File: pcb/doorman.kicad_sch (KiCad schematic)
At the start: 58 parts, among them J1 USB-C Connector, J2 Screw Terminals, J3 3V3 Test Pad, J4 Extension Board Connector, J5 Siedle BUS RX Test Pad, J6 BUS Test Pad, J7 BUS RX Test Pad, J8 TX Test Pad, J9 RX Test Pad, Q1 BC847BPN, Q2 BC817-40, Q3 BC817-40, Q4 BC817-40, Q5 BC807-40, Q6 BC807-40, SW1 Button, SW2 Button, U2 AP63203WU, U3 GAQY252G3S, U4 ESP32-S3-MINI-1

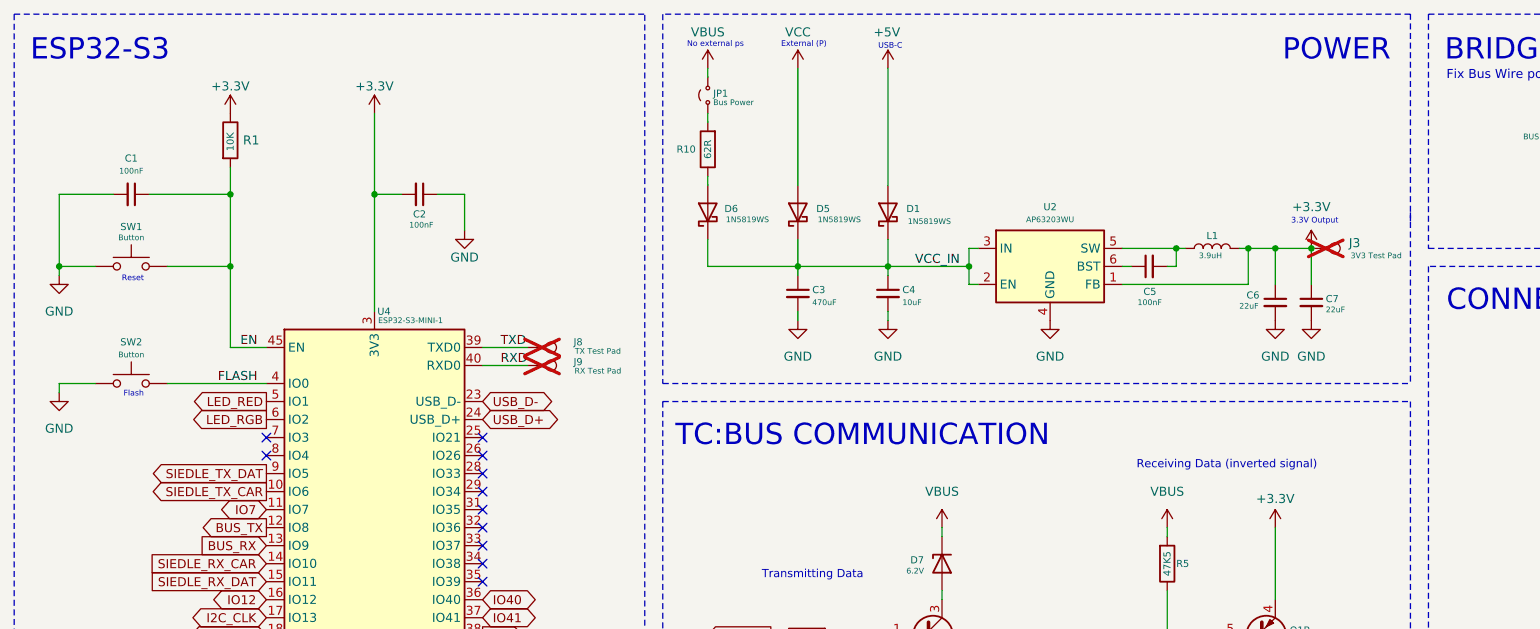
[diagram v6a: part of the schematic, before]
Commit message: WIP
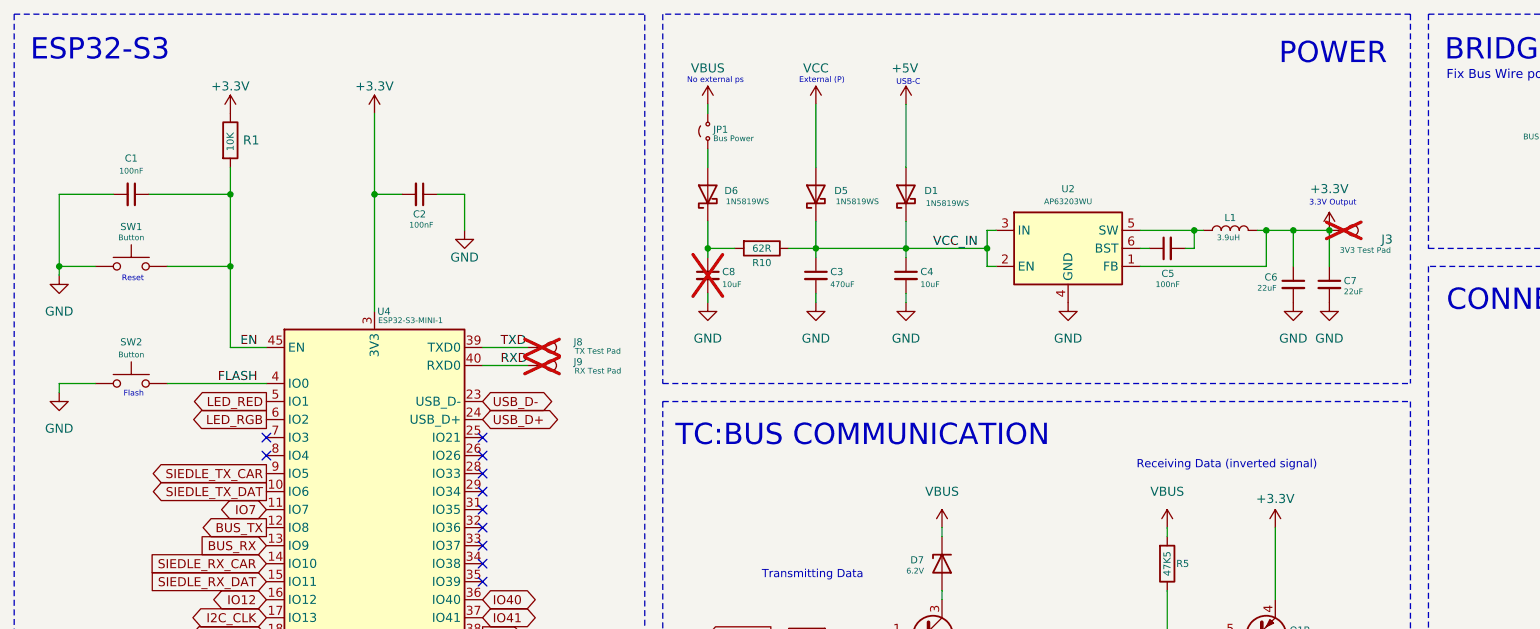
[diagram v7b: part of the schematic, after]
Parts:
- added C8: 10uF, Capacitor_SMD:C_1206_3216Metric, symbol Device:C_Small
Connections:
- net GND: now also C8.2
- net SIEDLE_TX_CAR: now also U4.9 (IO5); no longer U4.10 (IO6)
- net SIEDLE_TX_DAT: now also U4.10 (IO6); no longer U4.9 (IO5)
- net VCC_IN: now also R10.1; no longer D6.1 (K)
- net at D6.2 (A): now also JP1.1 (A); no longer R10.1
- net at R10.2: now also D6.1 (K), C8.1; no longer JP1.1 (A)
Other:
- moved on the sheet: C3, C4, C5, C6, C7, D1, D5, D6, J3, JP1, L1, R10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
